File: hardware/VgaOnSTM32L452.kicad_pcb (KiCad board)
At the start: 2 copper layers, 43.7 x 63.5 mm, 43 parts, among them J1 USB_B, J2 PS2_KEYBOARD, J3 VGA_OUT, P1 CONN_02X05, P2 PIN, P3 PIN, Q1 BC847, SW1 SW_Push, U1 STM32L452CUx, U2 TPS73033DBV, U3 SPI_NOR, Y1 8MHz

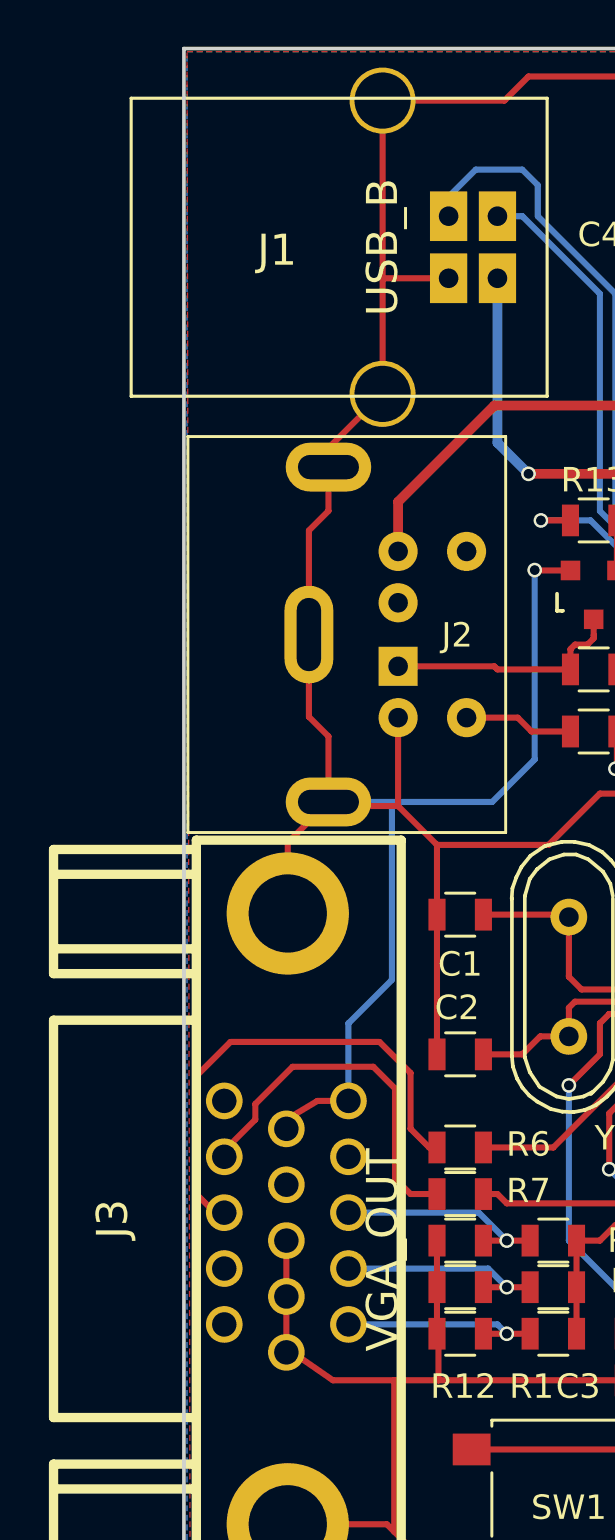
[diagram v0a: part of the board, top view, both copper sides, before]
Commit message: verze pro Kicad 5
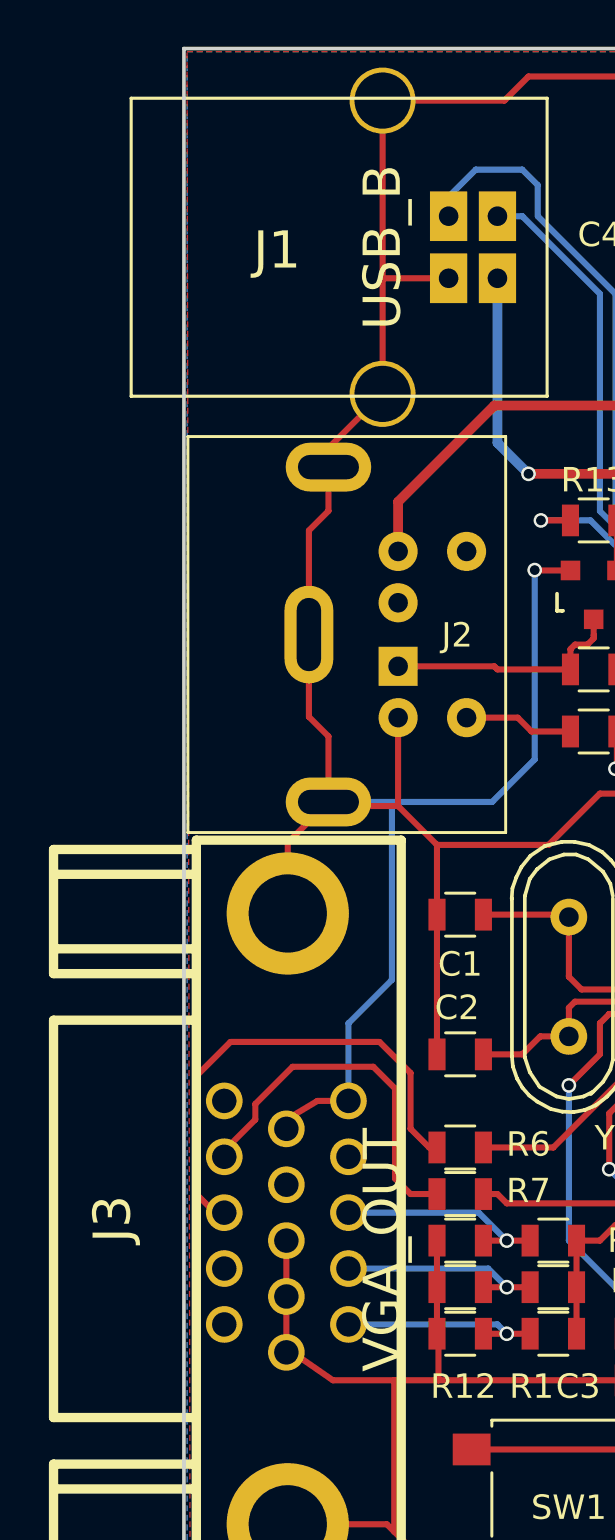
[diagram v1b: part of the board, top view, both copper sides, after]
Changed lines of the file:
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@@
-(kicad_pcb (version 4) (host pcbnew 4.0.7-e2-6376~58~ubuntu16.04.1)
+(kicad_pcb (version 20171130) (host pcbnew 5.0.2-bee76a0~70~ubuntu16.04.1)
   (general
-    (links 114)
-    (no_connects 0)
-    (area 116.256999 67.996999 160.095001 131.647001)
     (thickness 1.6)
     (drawings 7)
@@
     (pad_drill 0.762)
     (pad_to_mask_clearance 0.2)
+    (solder_mask_min_width 0.25)
     (aux_axis_origin 116.332 68.072)
     (grid_origin 116.332 68.072)
@@
       (layerselection 0x010e0_80000001)
       (usegerberextensions true)
+      (usegerberattributes false)
+      (usegerberadvancedattributes false)
+      (creategerberjobfile false)
       (excludeedgelayer true)
       (linewidth 0.100000)
@@
       (hpglpennumber 1)
       (hpglpenspeed 20)
-      (hpglpendiameter 15)
-      (hpglpenoverlay 2)
+      (hpglpendiameter 15.000000)
       (psnegative false)
       (psa4output false)
@@
       (drillshape 0)
       (scaleselection 1)
-      (outputdirectory fab))
+      (outputdirectory "fab"))
   )
   (net 0 "")
@@
     (descr "Crystal Quarz HC49/U vertical stehend")
     (tags "Crystal Quarz HC49/U vertical stehend")
-    (fp_text reference Y1 (at 6.604 -1.905 360) (layer F.SilkS)
-      (effects (font (size 1 1) (thickness 0.15)))
-    )
-    (fp_text value 8MHz (at 6.858 0.254 360) (layer F.Fab)
+    (fp_text reference Y1 (at 6.604 -1.905) (layer F.SilkS)
+      (effects (font (size 1 1) (thickness 0.15)))
+    )
+    (fp_text value 8MHz (at 6.858 0.254) (layer F.Fab)
       (effects (font (size 1 1) (thickness 0.15)))
     )
@@
       (net 2 GND))
     (model Capacitors_ThroughHole.3dshapes/C_Radial_D5_L6_P2.5.wrl
-      (at (xyz 0.0492126 0 0))
+      (offset (xyz 1.250000021226883 0 0))
       (scale (xyz 1 1 1))
       (rotate (xyz 0 0 90))
@@
     (tags "resistor 0805")
     (attr smd)
-    (fp_text reference C9 (at 2.794 -0.127 360) (layer F.SilkS)
+    (fp_text reference C9 (at 2.794 -0.127) (layer F.SilkS)
       (effects (font (size 1 1) (thickness 0.15)))
     )
@@
     (at 138.176 85.852 270)
     (attr smd)
-    (fp_text reference F1 (at 0 0 360) (layer F.SilkS)
-      (effects (font (size 1 1) (thickness 0.15)))
-    )
-    (fp_text value Polyfuse (at -0.127 -1.397 360) (layer F.Fab)
+    (fp_text reference F1 (at 0 0) (layer F.SilkS)
+      (effects (font (size 1 1) (thickness 0.15)))
+    )
+    (fp_text value Polyfuse (at -0.127 -1.397) (layer F.Fab)
       (effects (font (size 1 1) (thickness 0.15)))
     )
@@
     (at 124.46 76.2 270)
     (tags USB)
-    (fp_text reference J1 (at 0.127 4.318 360) (layer F.SilkS)
-      (effects (font (thickness 0.3048)))
+    (fp_text reference J1 (at 0.127 4.318) (layer F.SilkS)
+      (effects (font (size 1.524 1.524) (thickness 0.3048)))
     )
     (fp_text value USB_B (at 0 0 270) (layer F.SilkS)
-      (effects (font (thickness 0.3048)))
+      (effects (font (size 1.524 1.524) (thickness 0.3048)))
     )
     (fp_line (start -6.096 10.287) (end 6.096 10.287) (layer F.SilkS) (width 0.127))
@@
       (net 2 GND))
     (model connectors/USB_type_B.wrl
-      (at (xyz 0 0 0.001))
+      (offset (xyz 0 0 0.02539999961853028))
       (scale (xyz 0.3937 0.3937 0.3937))
       (rotate (xyz 0 0 0))
@@
     (descr "A footprint for the generic 6 pin Mini-DIN through hole connector with shell.")
     (tags "mini din 6pin connector socket")
-    (fp_text reference J2 (at -1.27 -2.413 360) (layer F.SilkS)
+    (fp_text reference J2 (at -1.27 -2.413) (layer F.SilkS)
       (effects (font (size 1 1) (thickness 0.15)))
     )
@@
     (descr SOT23-5)
     (attr smd)
-    (fp_text reference U2 (at 2.286 0.127 360) (layer F.SilkS)
+    (fp_text reference U2 (at 2.286 0.127) (layer F.SilkS)
       (effects (font (size 0.762 0.635) (thickness 0.127)))
     )
@@
     (descr "D-SUB 15 pin VGA socket, Tyco P/N 440467-1")
     (fp_text reference J3 (at 0 4.699 270) (layer F.SilkS)
-      (effects (font (thickness 0.3048)))
+      (effects (font (size 1.524 1.524) (thickness 0.3048)))
     )
     (fp_text value VGA_OUT (at 1.27 -6.35 270) (layer F.SilkS)
-      (effects (font (thickness 0.3048)))
+      (effects (font (size 1.524 1.524) (thickness 0.3048)))
     )
     (fp_line (start -10.033 1.27) (end -10.033 7.112) (layer F.SilkS) (width 0.381))
